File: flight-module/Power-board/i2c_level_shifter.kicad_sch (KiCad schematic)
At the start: 8 parts, among them J10 Pin Jumper, J9 Pin Jumper, Q5 NMOS, Q6 NMOS

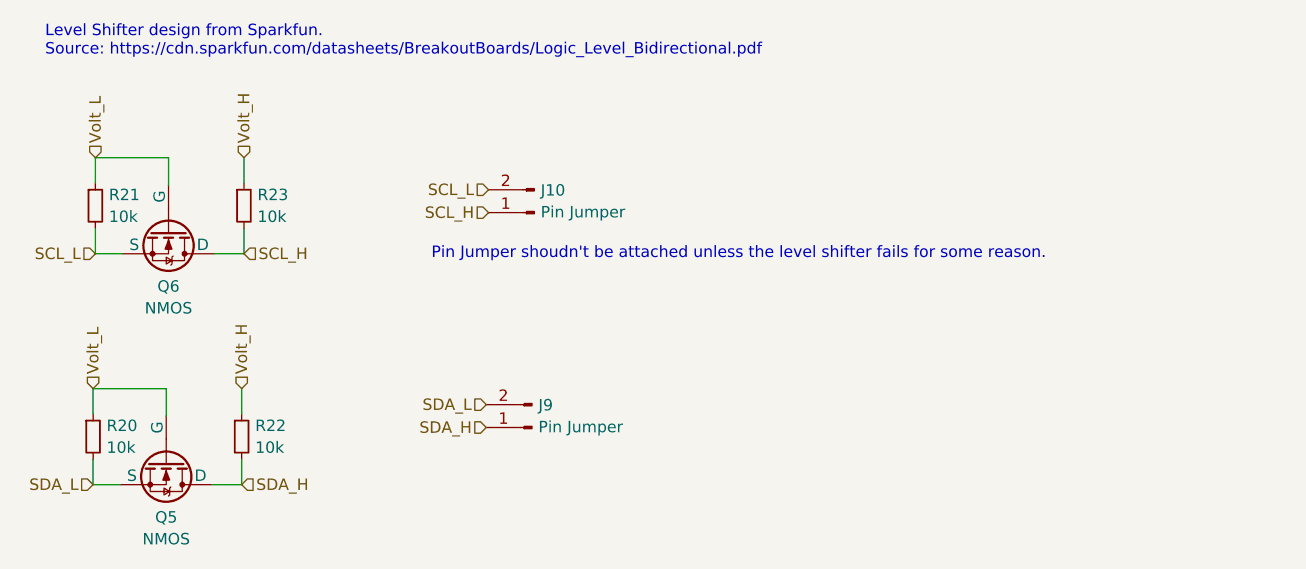
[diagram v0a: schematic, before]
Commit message: merge conflict fix
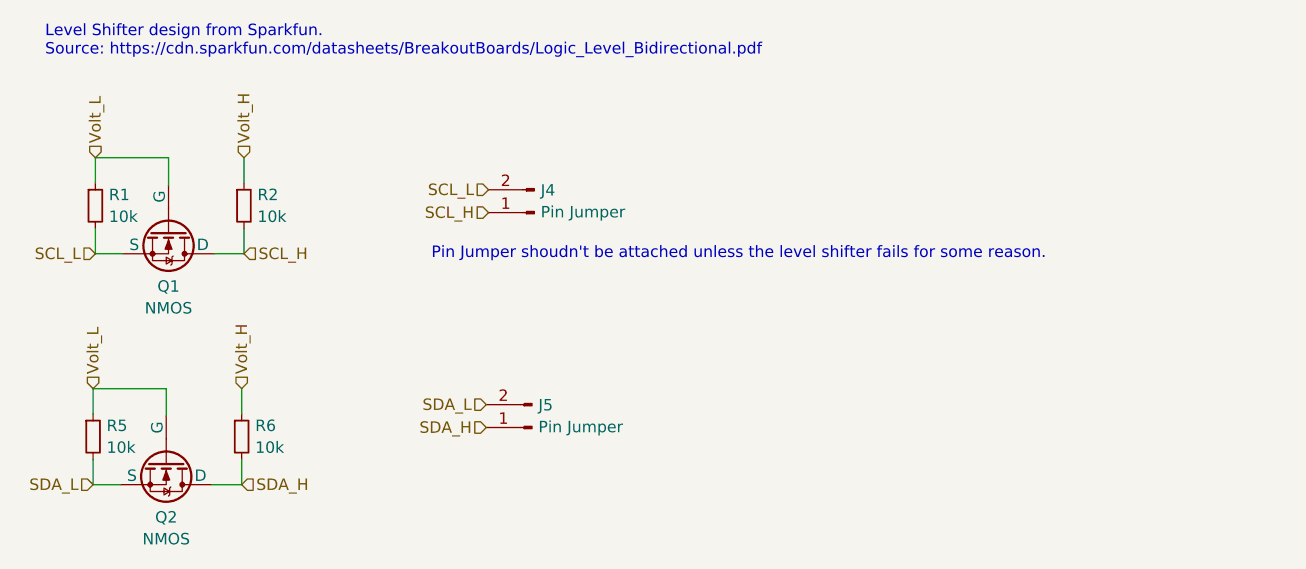
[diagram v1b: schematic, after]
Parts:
- renumbered J10 to J4, J9 to J5, Q6 to Q1, Q5 to Q2, R21 to R1, R23 to R2, R20 to R5, R22 to R6
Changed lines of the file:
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@@
   (symbol (lib_id "Device:R_Small") (at 108.712 125.984 0) (unit 1)
     (in_bom yes) (on_board yes) (dnp no) (fields_autoplaced)
-    (property "Reference" "R20" (at 110.2106 124.7719 0)
+    (property "Reference" "R5" (at 110.2106 124.7719 0)
       (effects (font (size 1.27 1.27)) (justify left))
     )
@@
       (project "Power-board"
         (path "/9e0a4b39-2b30-4bec-9684-92acf902e3a8/27658330-53e6-419c-8f56-73f4d9006175"
-          (reference "R20") (unit 1)
+          (reference "R5") (unit 1)
         )
       )
@@
   (symbol (lib_id "Simulation_SPICE:NMOS") (at 117.094 103.124 270) (unit 1)
     (in_bom yes) (on_board yes) (dnp no) (fields_autoplaced)
-    (property "Reference" "Q6" (at 117.094 109.2891 90)
+    (property "Reference" "Q1" (at 117.094 109.2891 90)
       (effects (font (size 1.27 1.27)))
     )
@@
       (project "Power-board"
         (path "/9e0a4b39-2b30-4bec-9684-92acf902e3a8/27658330-53e6-419c-8f56-73f4d9006175"
-          (reference "Q6") (unit 1)
+          (reference "Q1") (unit 1)
         )
       )
@@
   (symbol (lib_id "Device:R_Small") (at 108.966 100.33 0) (unit 1)
     (in_bom yes) (on_board yes) (dnp no) (fields_autoplaced)
-    (property "Reference" "R21" (at 110.4646 99.1179 0)
+    (property "Reference" "R1" (at 110.4646 99.1179 0)
       (effects (font (size 1.27 1.27)) (justify left))
     )
@@
       (project "Power-board"
         (path "/9e0a4b39-2b30-4bec-9684-92acf902e3a8/27658330-53e6-419c-8f56-73f4d9006175"
-          (reference "R21") (unit 1)
+          (reference "R1") (unit 1)
         )
       )
@@
   (symbol (lib_id "Device:R_Small") (at 125.222 125.984 0) (unit 1)
     (in_bom yes) (on_board yes) (dnp no) (fields_autoplaced)
-    (property "Reference" "R22" (at 126.7206 124.7719 0)
+    (property "Reference" "R6" (at 126.7206 124.7719 0)
       (effects (font (size 1.27 1.27)) (justify left))
     )
@@
       (project "Power-board"
         (path "/9e0a4b39-2b30-4bec-9684-92acf902e3a8/27658330-53e6-419c-8f56-73f4d9006175"
-          (reference "R22") (unit 1)
+          (reference "R6") (unit 1)
         )
       )
@@
   (symbol (lib_id "Connector:Conn_01x02_Pin") (at 157.734 101.092 180) (unit 1)
     (in_bom yes) (on_board yes) (dnp no) (fields_autoplaced)
-    (property "Reference" "J10" (at 158.4452 98.6099 0)
+    (property "Reference" "J4" (at 158.4452 98.6099 0)
       (effects (font (size 1.27 1.27)) (justify right))
     )
@@
       (project "Power-board"
         (path "/9e0a4b39-2b30-4bec-9684-92acf902e3a8/27658330-53e6-419c-8f56-73f4d9006175"
-          (reference "J10") (unit 1)
+          (reference "J4") (unit 1)
         )
       )
@@
   (symbol (lib_id "Device:R_Small") (at 125.476 100.33 0) (unit 1)
     (in_bom yes) (on_board yes) (dnp no) (fields_autoplaced)
-    (property "Reference" "R23" (at 126.9746 99.1179 0)
+    (property "Reference" "R2" (at 126.9746 99.1179 0)
       (effects (font (size 1.27 1.27)) (justify left))
     )
@@
       (project "Power-board"
         (path "/9e0a4b39-2b30-4bec-9684-92acf902e3a8/27658330-53e6-419c-8f56-73f4d9006175"
-          (reference "R23") (unit 1)
+          (reference "R2") (unit 1)
         )
       )
@@
   (symbol (lib_id "Connector:Conn_01x02_Pin") (at 157.48 124.968 180) (unit 1)
     (in_bom yes) (on_board yes) (dnp no) (fields_autoplaced)
-    (property "Reference" "J9" (at 158.1912 122.4859 0)
+    (property "Reference" "J5" (at 158.1912 122.4859 0)
       (effects (font (size 1.27 1.27)) (justify right))
     )
@@
       (project "Power-board"
         (path "/9e0a4b39-2b30-4bec-9684-92acf902e3a8/27658330-53e6-419c-8f56-73f4d9006175"
-          (reference "J9") (unit 1)
+          (reference "J5") (unit 1)
         )
       )
@@
   (symbol (lib_id "Simulation_SPICE:NMOS") (at 116.84 128.778 270) (unit 1)
     (in_bom yes) (on_board yes) (dnp no) (fields_autoplaced)
-    (property "Reference" "Q5" (at 116.84 134.9431 90)
+    (property "Reference" "Q2" (at 116.84 134.9431 90)
       (effects (font (size 1.27 1.27)))
     )
@@
       (project "Power-board"
         (path "/9e0a4b39-2b30-4bec-9684-92acf902e3a8/27658330-53e6-419c-8f56-73f4d9006175"
-          (reference "Q5") (unit 1)
-        )
-      )
+          (reference "Q2") (unit 1)
+        )
+      )

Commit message: update on flight pcbs
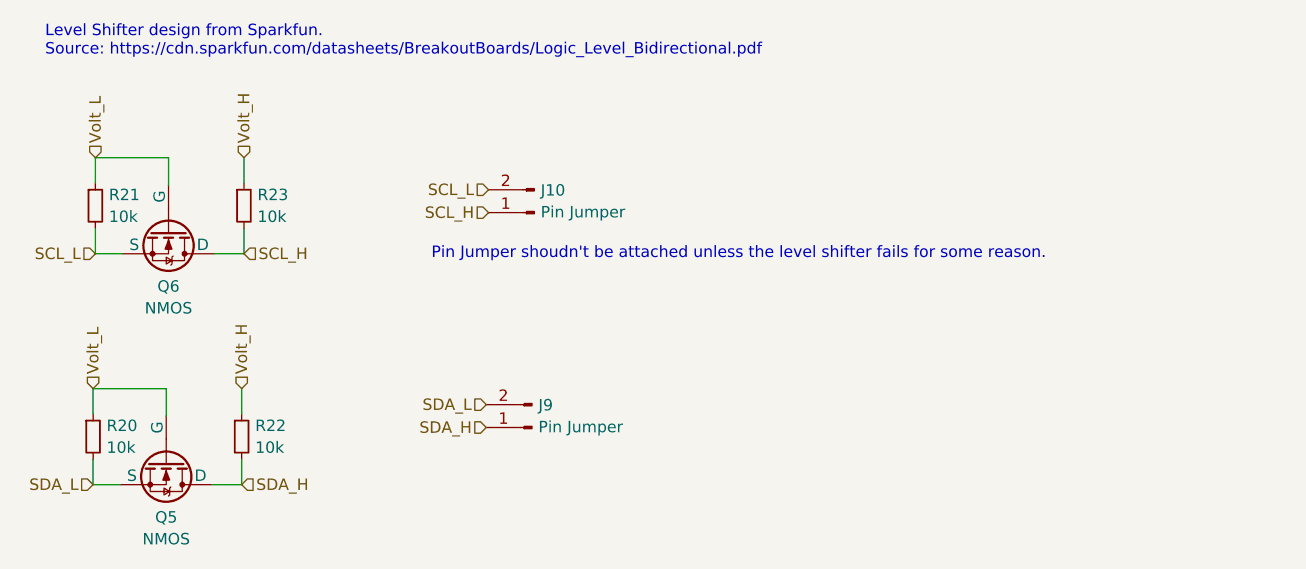
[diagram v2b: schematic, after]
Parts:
- renumbered J4 to J10, J5 to J9, Q2 to Q5, Q1 to Q6, R5 to R20, R1 to R21, R6 to R22, R2 to R23
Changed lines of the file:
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@@
   (symbol (lib_id "Device:R_Small") (at 108.712 125.984 0) (unit 1)
     (in_bom yes) (on_board yes) (dnp no) (fields_autoplaced)
-    (property "Reference" "R5" (at 110.2106 124.7719 0)
+    (property "Reference" "R20" (at 110.2106 124.7719 0)
       (effects (font (size 1.27 1.27)) (justify left))
     )
@@
       (project "Power-board"
         (path "/9e0a4b39-2b30-4bec-9684-92acf902e3a8/27658330-53e6-419c-8f56-73f4d9006175"
-          (reference "R5") (unit 1)
+          (reference "R20") (unit 1)
         )
       )
@@
   (symbol (lib_id "Simulation_SPICE:NMOS") (at 117.094 103.124 270) (unit 1)
     (in_bom yes) (on_board yes) (dnp no) (fields_autoplaced)
-    (property "Reference" "Q1" (at 117.094 109.2891 90)
+    (property "Reference" "Q6" (at 117.094 109.2891 90)
       (effects (font (size 1.27 1.27)))
     )
@@
       (project "Power-board"
         (path "/9e0a4b39-2b30-4bec-9684-92acf902e3a8/27658330-53e6-419c-8f56-73f4d9006175"
-          (reference "Q1") (unit 1)
+          (reference "Q6") (unit 1)
         )
       )
@@
   (symbol (lib_id "Device:R_Small") (at 108.966 100.33 0) (unit 1)
     (in_bom yes) (on_board yes) (dnp no) (fields_autoplaced)
-    (property "Reference" "R1" (at 110.4646 99.1179 0)
+    (property "Reference" "R21" (at 110.4646 99.1179 0)
       (effects (font (size 1.27 1.27)) (justify left))
     )
@@
       (project "Power-board"
         (path "/9e0a4b39-2b30-4bec-9684-92acf902e3a8/27658330-53e6-419c-8f56-73f4d9006175"
-          (reference "R1") (unit 1)
+          (reference "R21") (unit 1)
         )
       )
@@
   (symbol (lib_id "Device:R_Small") (at 125.222 125.984 0) (unit 1)
     (in_bom yes) (on_board yes) (dnp no) (fields_autoplaced)
-    (property "Reference" "R6" (at 126.7206 124.7719 0)
+    (property "Reference" "R22" (at 126.7206 124.7719 0)
       (effects (font (size 1.27 1.27)) (justify left))
     )
@@
       (project "Power-board"
         (path "/9e0a4b39-2b30-4bec-9684-92acf902e3a8/27658330-53e6-419c-8f56-73f4d9006175"
-          (reference "R6") (unit 1)
+          (reference "R22") (unit 1)
         )
       )
@@
   (symbol (lib_id "Connector:Conn_01x02_Pin") (at 157.734 101.092 180) (unit 1)
     (in_bom yes) (on_board yes) (dnp no) (fields_autoplaced)
-    (property "Reference" "J4" (at 158.4452 98.6099 0)
+    (property "Reference" "J10" (at 158.4452 98.6099 0)
       (effects (font (size 1.27 1.27)) (justify right))
     )
@@
       (project "Power-board"
         (path "/9e0a4b39-2b30-4bec-9684-92acf902e3a8/27658330-53e6-419c-8f56-73f4d9006175"
-          (reference "J4") (unit 1)
+          (reference "J10") (unit 1)
         )
       )
@@
   (symbol (lib_id "Device:R_Small") (at 125.476 100.33 0) (unit 1)
     (in_bom yes) (on_board yes) (dnp no) (fields_autoplaced)
-    (property "Reference" "R2" (at 126.9746 99.1179 0)
+    (property "Reference" "R23" (at 126.9746 99.1179 0)
       (effects (font (size 1.27 1.27)) (justify left))
     )
@@
       (project "Power-board"
         (path "/9e0a4b39-2b30-4bec-9684-92acf902e3a8/27658330-53e6-419c-8f56-73f4d9006175"
-          (reference "R2") (unit 1)
+          (reference "R23") (unit 1)
         )
       )
@@
   (symbol (lib_id "Connector:Conn_01x02_Pin") (at 157.48 124.968 180) (unit 1)
     (in_bom yes) (on_board yes) (dnp no) (fields_autoplaced)
-    (property "Reference" "J5" (at 158.1912 122.4859 0)
+    (property "Reference" "J9" (at 158.1912 122.4859 0)
       (effects (font (size 1.27 1.27)) (justify right))
     )
@@
       (project "Power-board"
         (path "/9e0a4b39-2b30-4bec-9684-92acf902e3a8/27658330-53e6-419c-8f56-73f4d9006175"
-          (reference "J5") (unit 1)
+          (reference "J9") (unit 1)
         )
       )
@@
   (symbol (lib_id "Simulation_SPICE:NMOS") (at 116.84 128.778 270) (unit 1)
     (in_bom yes) (on_board yes) (dnp no) (fields_autoplaced)
-    (property "Reference" "Q2" (at 116.84 134.9431 90)
+    (property "Reference" "Q5" (at 116.84 134.9431 90)
       (effects (font (size 1.27 1.27)))
     )
@@
       (project "Power-board"
         (path "/9e0a4b39-2b30-4bec-9684-92acf902e3a8/27658330-53e6-419c-8f56-73f4d9006175"
-          (reference "Q2") (unit 1)
-        )
-      )
+          (reference "Q5") (unit 1)
+        )
+      )
